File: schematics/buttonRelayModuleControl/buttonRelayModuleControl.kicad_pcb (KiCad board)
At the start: 2 copper layers, 68.8 x 37.3 mm, 20 parts, among them J1 Conn_AC_MAINS, J2 Programmer, SW1 SW_Push_LED, SW2 SW_Push_LED, U2 TSP-05, U3 ATmega328PB-AU

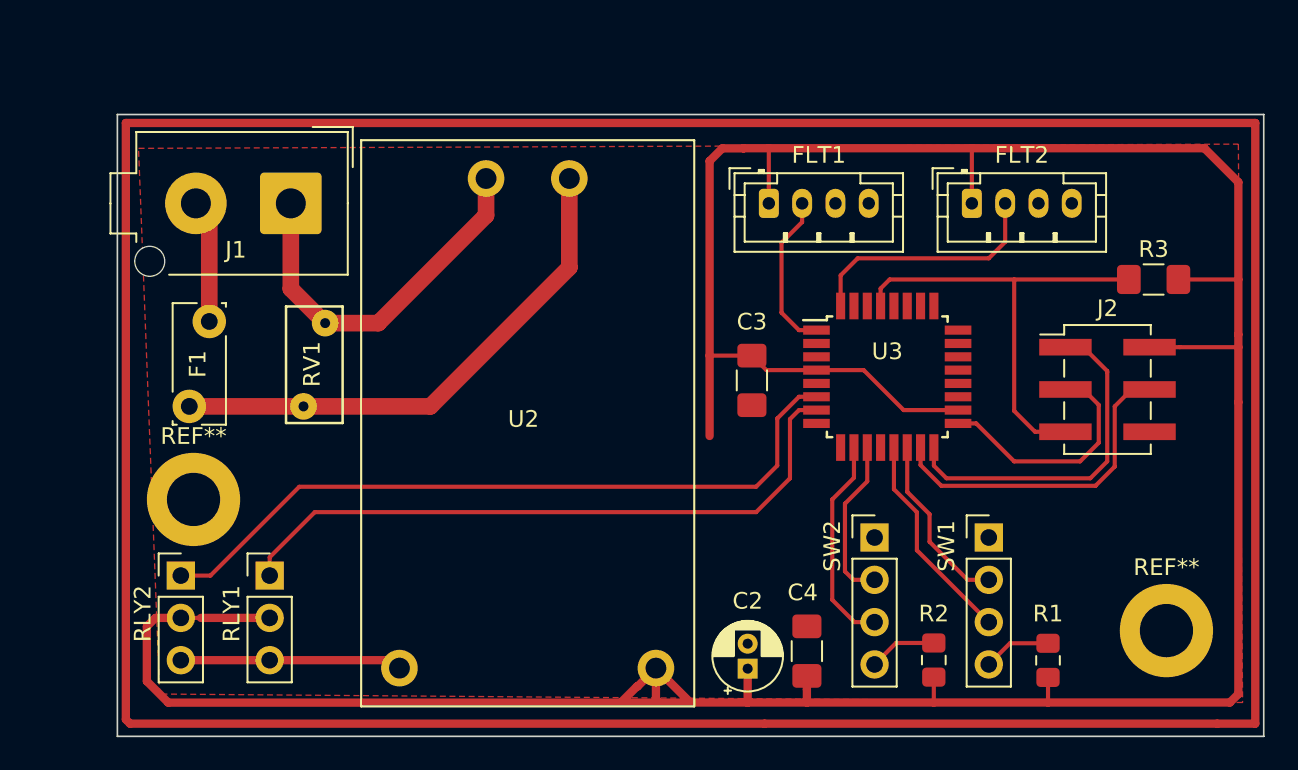
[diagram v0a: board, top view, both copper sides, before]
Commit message: Initial Firmware
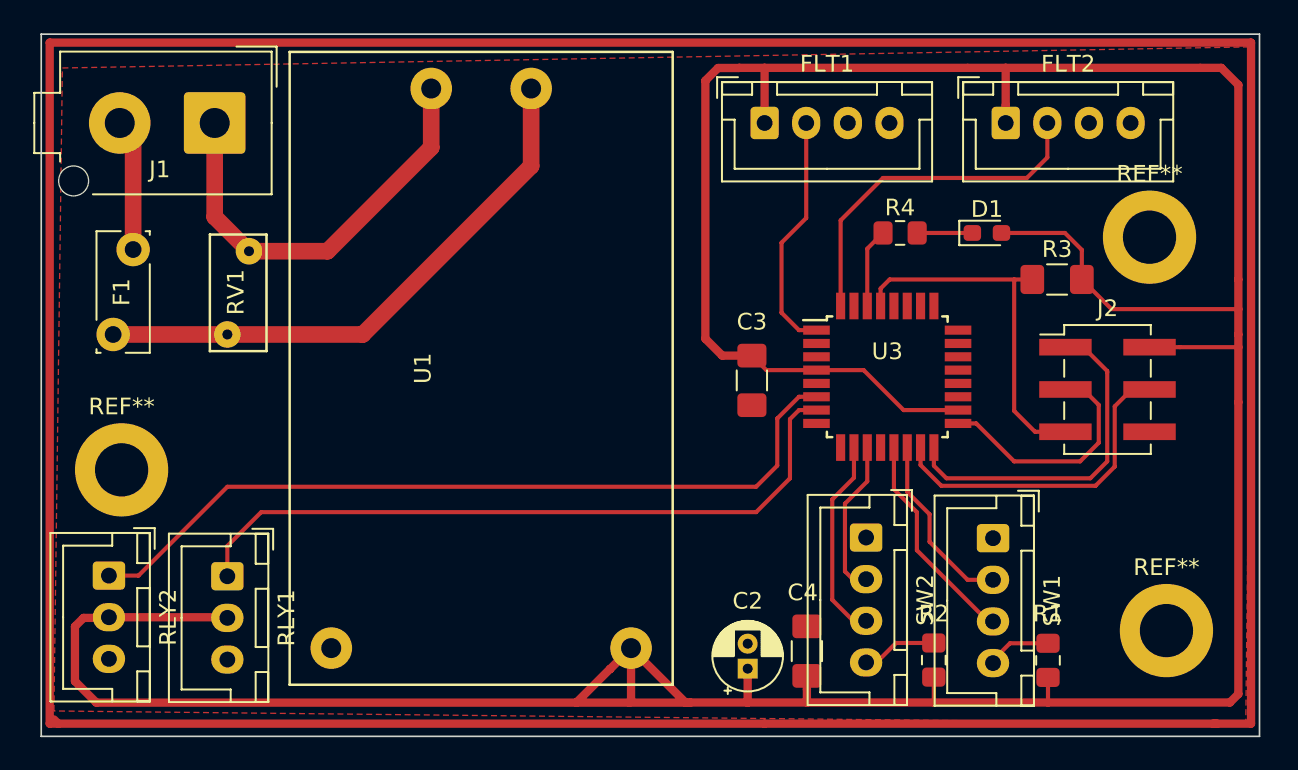
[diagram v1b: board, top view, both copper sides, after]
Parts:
- removed U2: TSP-05, Power_Supply:HLK-PM05
- added D1: LED, LED_SMD:LED_0603_1608Metric_Pad1.05x0.95mm_HandSolder, F.Cu at (159.4, 85.3)
- added R4: 1k, Resistor_SMD:R_0805_2012Metric_Pad1.15x1.40mm_HandSolder, F.Cu at (154.2, 85.3)
- added REF**: MountingHole_3.2mm_M3_DIN965_Pad, MountingHole:MountingHole_3.2mm_M3_DIN965_Pad, F.Cu at (169.2, 85.6)
- added U1: HLK-5M05, remoteSwitch_footprints:HLK-5M05, F.Cu at (129.0, 93.5)
- FLT1, FLT2: footprint Connectors_JST:JST_PH_B4B-PH-K_1x04_P2.00mm_Vertical -> Connector_JST:JST_XH_B04B-XH-A_1x04_P2.50mm_Vertical
- RLY1, RLY2: footprint Connector_PinHeader_2.54mm:PinHeader_1x03_P2.54mm_Vertical -> Connector_JST:JST_XH_B03B-XH-A_1x03_P2.50mm_Vertical
- SW1, SW2: footprint Connector_PinHeader_2.54mm:PinHeader_1x04_P2.54mm_Vertical -> Connector_JST:JST_XH_B04B-XH-A_1x04_P2.50mm_Vertical
- moved J1 6.65 mm to (113.0, 78.7)
- moved F1 6.29 mm to (106.9, 91.4)
- moved RV1 6.29 mm to (113.8, 91.4)
- moved R3 5.80 mm to (163.6, 88.1)
- moved FLT2 5.24 mm to (160.5, 78.7)
- moved FLT1 4.83 mm to (146.1, 78.7)
- moved REF** 4.67 mm to (107.4, 99.6)
- moved RLY2 4.32 mm to (106.7, 105.9), turned to 270 degrees
- moved RLY1 2.54 mm to (113.8, 106.0), turned to 270 degrees
- moved SW2 0.51 mm to (152.1, 103.6), turned to 270 degrees
- moved SW1 0.26 mm to (159.8, 103.7), turned to 270 degrees
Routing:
- net +5V: track 204.5 -> 233.4 mm
- net (no net): track 207.6 -> 226.7 mm
- net GND: track 13.3 -> 0.00 mm
- net /SENS2: track 14.9 -> 21.2 mm
- net /RESET: track 27.7 -> 21.9 mm
- net /SENS1: track 10.1 -> 15.1 mm
- net Net-(R4-Pad2): track 0.00 -> 4.78 mm
- net /RELAY2: track 44.3 -> 48.6 mm
- net Net-(D1-Pad1): track 0.00 -> 3.31 mm
- net Net-(J1-Pad1): track 22.6 -> 25.6 mm
- net /RELAY1: track 39.7 -> 42.7 mm
- net Net-(F1-Pad1): track 31.6 -> 33.9 mm
- net Net-(F1-Pad2): track 7.43 -> 7.93 mm
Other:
- board size 68.8 x 37.3 mm -> 73.2 x 42.2 mm
